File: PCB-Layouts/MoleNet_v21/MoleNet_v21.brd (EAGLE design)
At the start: 76.5 x 67.6 mm, 33 parts, among them IC1 25LC080P, Q1 BS250, Q2 BS170, U1 MCP1703-5002E/DB, U2 ATMEGA328P-PU, U3 RFM69CW, X1 SMA-142-0711-821/826

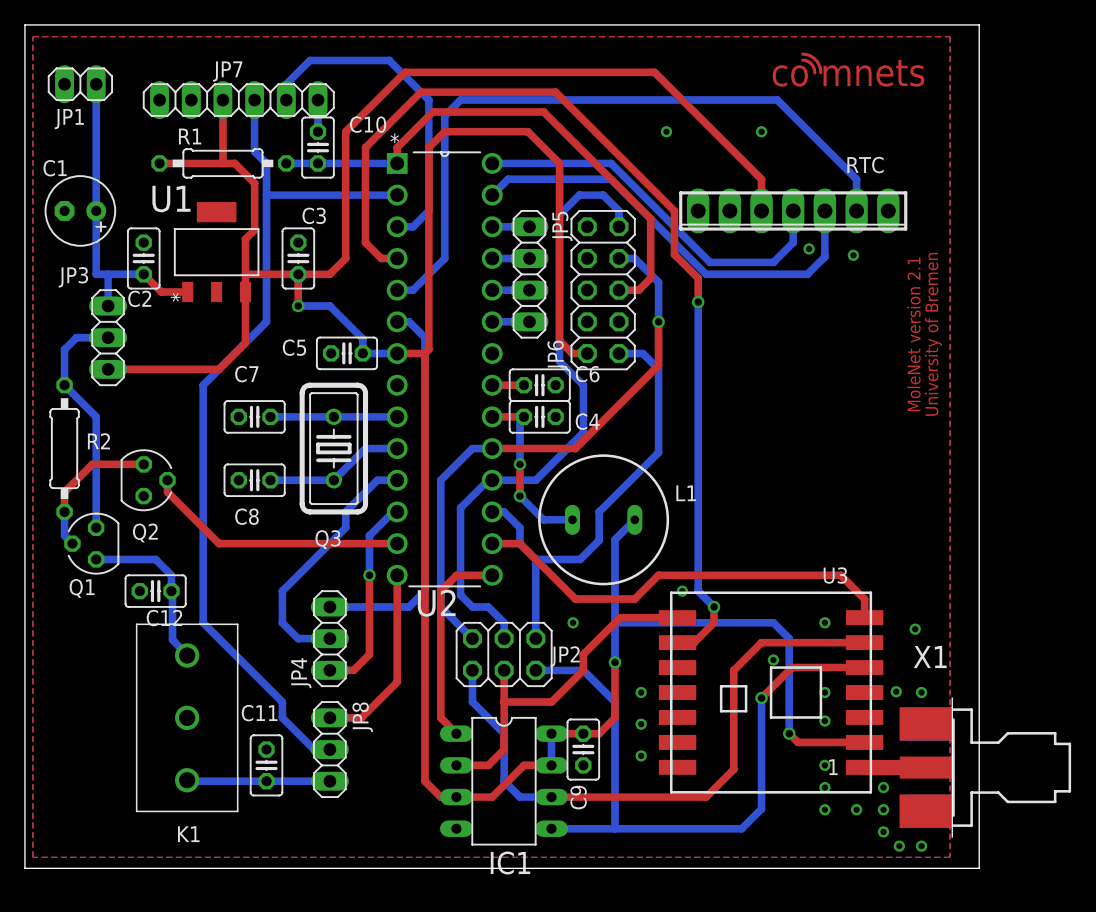
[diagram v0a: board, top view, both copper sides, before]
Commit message: MoleNet version 2.1 rtm
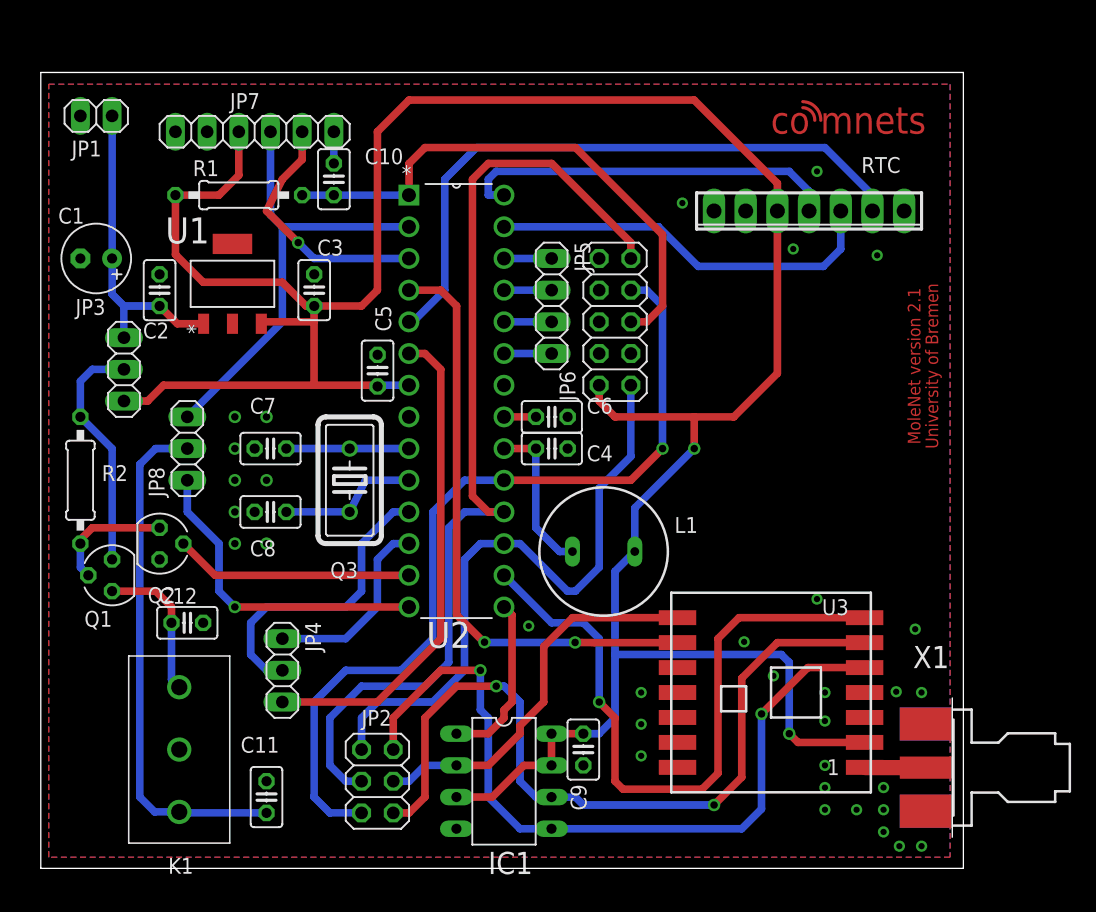
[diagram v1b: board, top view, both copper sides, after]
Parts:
- moved JP8 26.7 mm to (12.7, 33.0), turned to 90 degrees
- moved JP2 14.4 mm to (27.9, 6.35), turned to 270 degrees
- moved Q2 5.24 mm to (10.5, 25.4)
- moved JP4 4.58 mm to (20.3, 15.2), turned to 270 degrees
- moved C1 4.02 mm to (5.40, 48.3)
- moved C12 3.59 mm to (12.7, 19.1), turned to 0 degrees
- moved JP5 3.10 mm to (41.9, 44.5)
- moved R2 2.84 mm to (4.13, 30.5)
- moved Q3 2.84 mm to (25.7, 30.5)
- moved C10 2.84 mm to (24.4, 54.6)
- moved JP3 2.84 mm to (7.62, 39.4)
- moved Q1 2.84 mm to (6.67, 22.9)
- moved R1 2.84 mm to (16.8, 53.3)
- moved U1 2.84 mm to (16.3, 46.2)
- moved C2 2.84 mm to (10.5, 45.7)
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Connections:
- net RXD: now also JP8.3; no longer JP8.2
- net SENSRXD: now also JP8.2; no longer JP8.3
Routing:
- net VCC: track 258.2 -> 217.7 mm, vias 3 -> 2
- net RXD: track 70.0 -> 36.6 mm
- net D2: track 79.2 -> 47.7 mm
- net SENSRXD: track 11.5 -> 41.7 mm
- net MISO: track 50.5 -> 79.6 mm
- net SCK: track 45.7 -> 68.8 mm
- net NSS: track 34.8 -> 54.0 mm, vias 0 -> 1
- net SCKSW: track 49.1 -> 63.4 mm, vias 0 -> 2
- net MOSI: track 37.3 -> 50.6 mm
- net D8: track 15.2 -> 25.7 mm, vias 0 -> 1
- net MOSISW: track 53.2 -> 62.6 mm, vias 1 -> 2
- net D4: track 31.2 -> 39.5 mm
- net TXD: track 26.8 -> 20.3 mm, vias 0 -> 1
- net D3: track 55.0 -> 51.0 mm
- net D5: track 20.5 -> 24.2 mm
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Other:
- board size 76.5 x 67.6 mm -> 74 x 63.8 mm
